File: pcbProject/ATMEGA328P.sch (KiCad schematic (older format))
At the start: 8 parts, among them SW1 RESET_SWITCH, U2 ATmega328P-AU, Y1 CSTCE16MOV53-R0

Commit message: bijna klaar pcb
nog enkele andere planes toevoegen
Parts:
- SW1: footprint Button_Switch_SMD:SW_SPST_PTS645 -> eigenfootprint:SW_SPST_PTS645_aangepast
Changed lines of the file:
@@
 F 0 "SW1" V 1350 2725 60  0000 C CNN
 F 1 "RESET_SWITCH" V 1650 2975 60  0000 C CNN
-F 2 "Button_Switch_SMD:SW_SPST_PTS645" H 1500 2425 60  0001 C CNN
+F 2 "eigenfootprint:SW_SPST_PTS645_aangepast" H 1500 2425 60  0001 C CNN
 F 3 "http://industrial.panasonic.com/www-data/pdf/ATK0000/ATK0000CE28.pdf" H 1500 2425 60  0001 C CNN
 F 4 "SWITCH TACTILE SPST-NO 0.02A 15V" H 1500 2425 60  0001 C CNN "Characteristics"

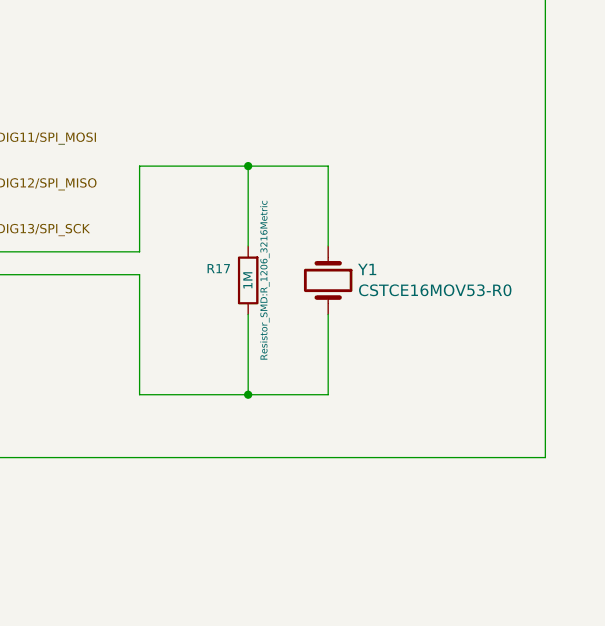
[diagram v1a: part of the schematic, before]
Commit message: NIEUWE PCB VERSIE
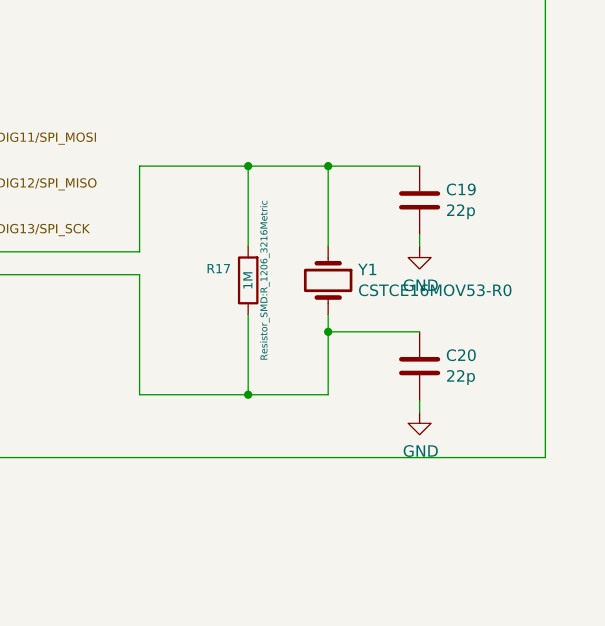
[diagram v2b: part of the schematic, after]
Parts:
- added C19, C20: 22p, Capacitor_SMD:C_0805_2012Metric, symbol Device:C
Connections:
- net GND: now also C19.2, C20.2
- net at R17.1, U2.8 (XTAL2/PB7), Y1.2: now also C20.1
- net at R17.2, U2.7 (XTAL1/PB6), Y1.1: now also C19.1
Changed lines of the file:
@@
 $EndComp
 Wire Wire Line
-	9950 3625 9950 3975
+	9950 3625 9950 3700
 Wire Wire Line
 	9950 2975 9950 3325
+$Comp
+L Device:C C20
+U 1 1 5C89A715
+P 10350 3850
+F 0 "C20" H 10465 3896 50  0000 L CNN
+F 1 "22p" H 10465 3805 50  0000 L CNN
+F 2 "Capacitor_SMD:C_0805_2012Metric" H 10388 3700 50  0001 C CNN
+F 3 "~" H 10350 3850 50  0001 C CNN
+	1    10350 3850
+	1    0    0    -1
+$EndComp
+$Comp
+L Device:C C19
+U 1 1 5C89A779
+P 10350 3125
+F 0 "C19" H 10465 3171 50  0000 L CNN
+F 1 "22p" H 10465 3080 50  0000 L CNN
+F 2 "Capacitor_SMD:C_0805_2012Metric" H 10388 2975 50  0001 C CNN
+F 3 "~" H 10350 3125 50  0001 C CNN
+	1    10350 3125
+	1    0    0    -1
+$EndComp
+Wire Wire Line
+	9950 2975 10350 2975
+Connection ~ 9950 2975
+Wire Wire Line
+	9950 3700 10350 3700
+Connection ~ 9950 3700
+Wire Wire Line
+	9950 3700 9950 3975
+$Comp
+L power:GND #PWR09
+U 1 1 5C89ED8F
+P 10350 4050
+F 0 "#PWR09" H 10350 3800 50  0001 C CNN
+F 1 "GND" H 10355 3877 50  0000 C CNN
+F 2 "" H 10350 4050 50  0001 C CNN
+F 3 "" H 10350 4050 50  0001 C CNN
+	1    10350 4050
+	1    0    0    -1
+$EndComp
+$Comp
+L power:GND #PWR08
+U 1 1 5C89EDC5
+P 10350 3325
+F 0 "#PWR08" H 10350 3075 50  0001 C CNN
+F 1 "GND" H 10355 3152 50  0000 C CNN
+F 2 "" H 10350 3325 50  0001 C CNN
+F 3 "" H 10350 3325 50  0001 C CNN
+	1    10350 3325
+	1    0    0    -1
+$EndComp
+Wire Wire Line
+	10350 3325 10350 3275
+Wire Wire Line
+	10350 4050 10350 4000
 $EndSCHEMATC
